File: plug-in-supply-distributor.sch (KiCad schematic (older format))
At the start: 35 parts, among them J1 Conn_02x18_Odd_Even, J2 Conn_02x04_Odd_Even, J3 PV-3, J4 PV-3, J5 PV-3, Q1 2N7002K, Q2 SUD50P04-08, Q3 2N7002K, Q4 SUD50P04-08, U1 74LS27, U2 BD450M5FP

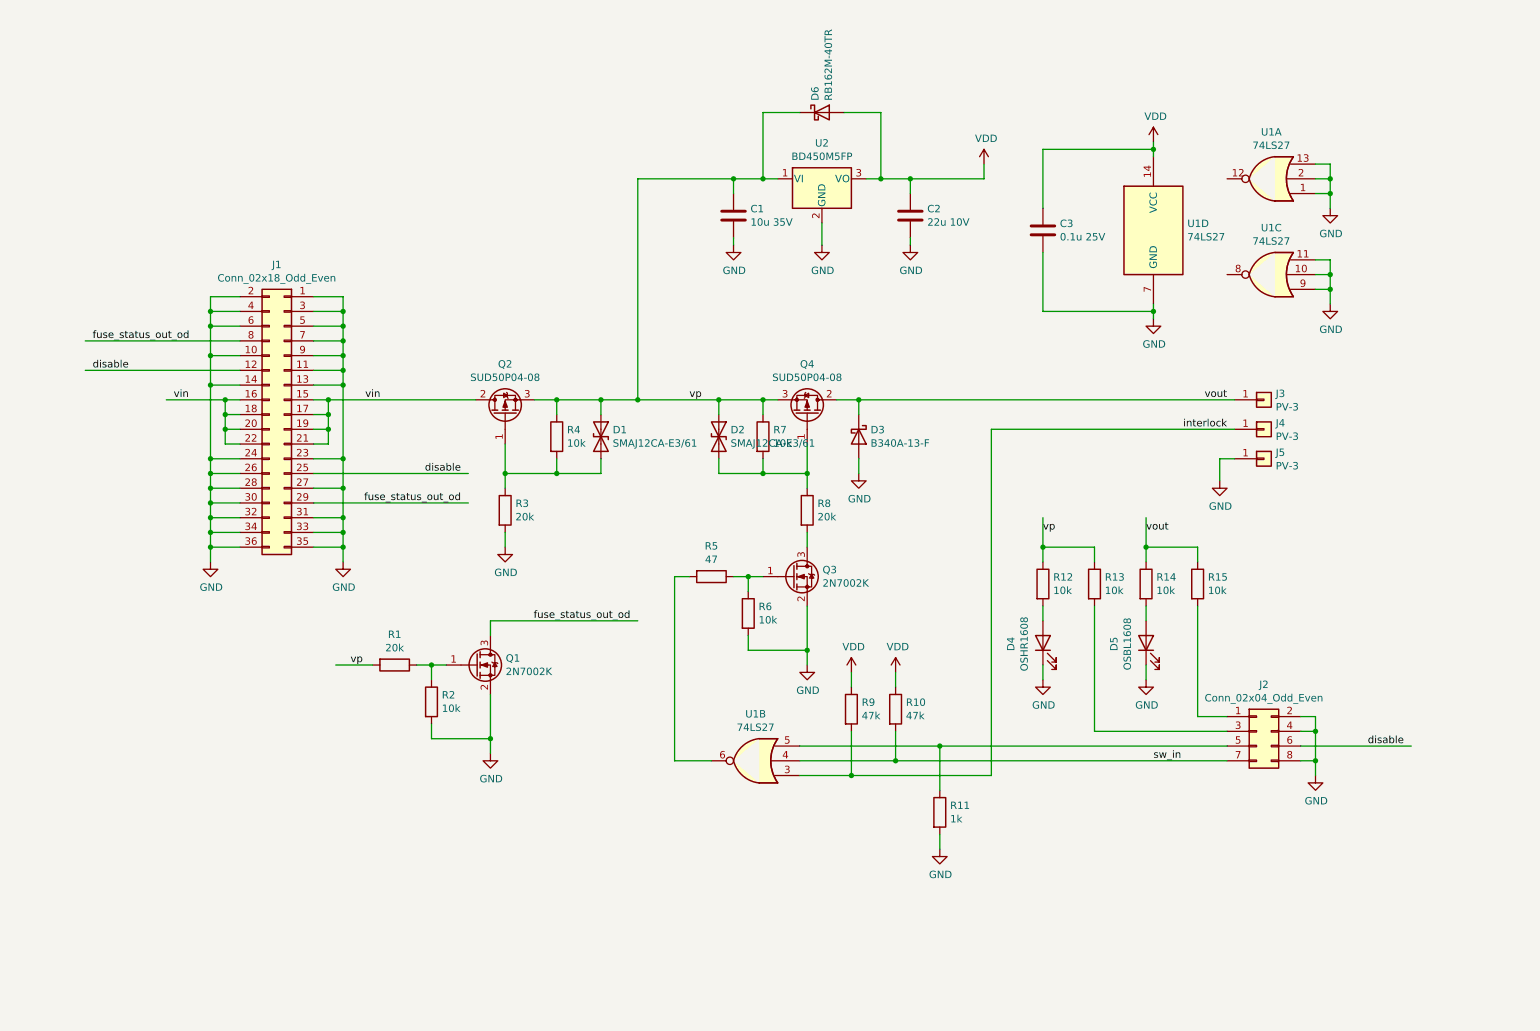
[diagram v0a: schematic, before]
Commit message: Update kicad files
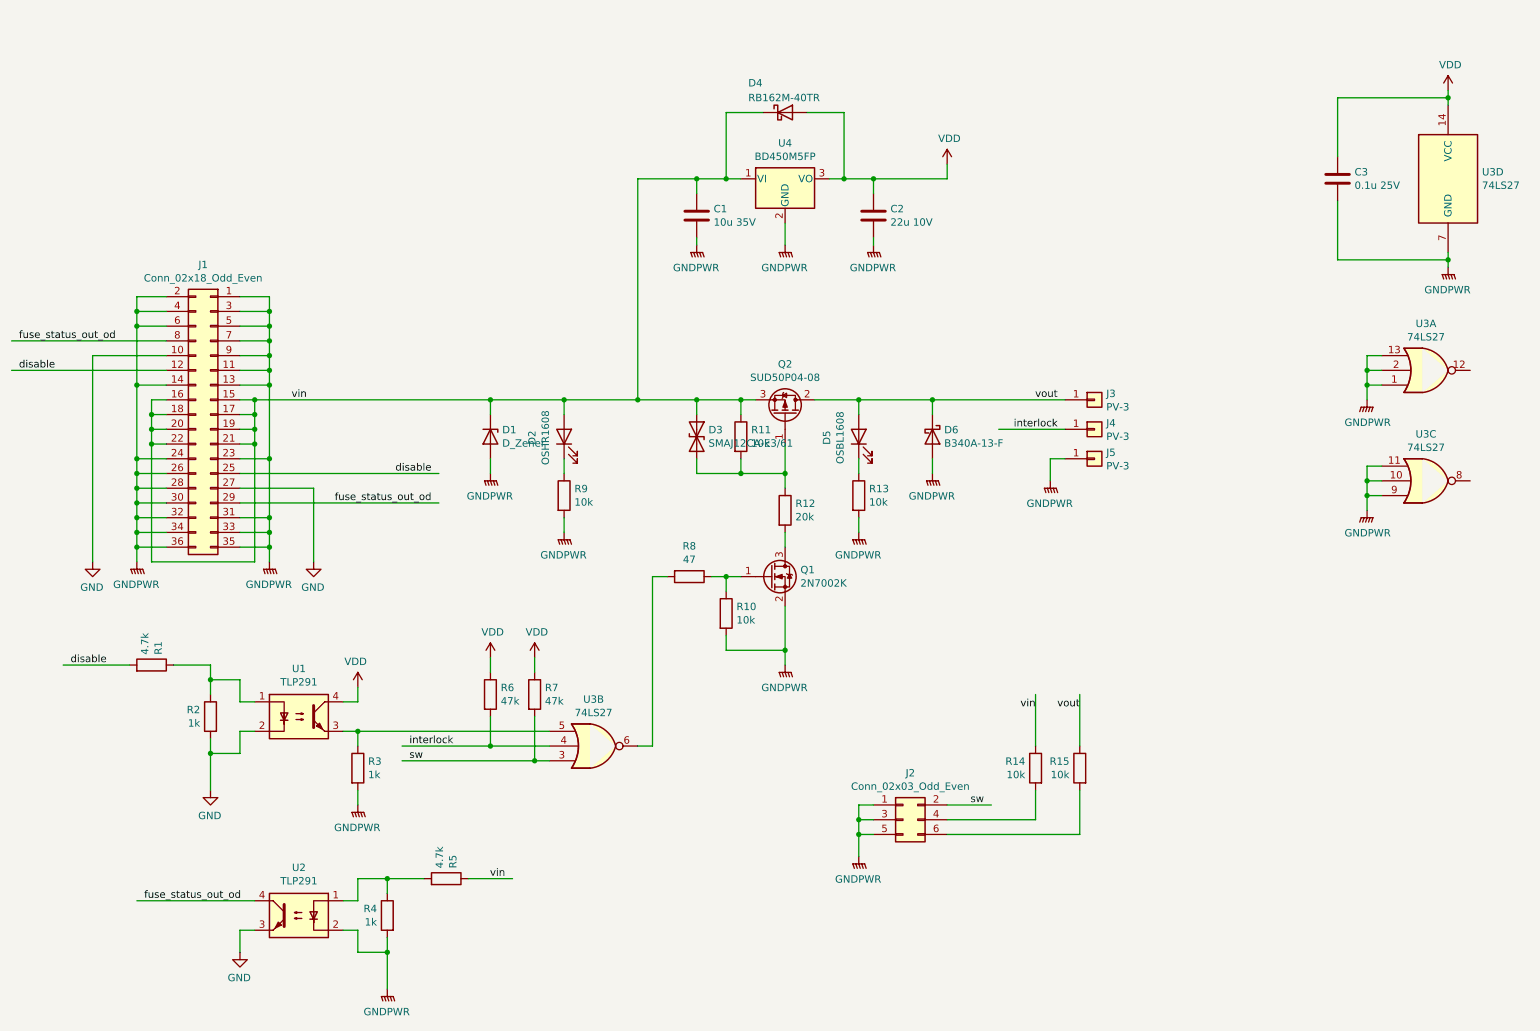
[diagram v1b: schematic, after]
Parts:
- removed D1: SMAJ12CA-E3/61, Diode_SMD:D_SMA, symbol Device:D_TVS
- removed J2: Conn_02x04_Odd_Even, Connector_PinHeader_2.54mm:PinHeader_2x04_P2.54mm_Horizontal, symbol Connector_Generic:Conn_02x04_Odd_Even
- removed Q1: 2N7002K, Package_TO_SOT_SMD:SOT-23, symbol Transistor_FET:2N7002K
- removed Q2: SUD50P04-08, Package_TO_SOT_SMD:TO-252-2, symbol Transistor_FET:SUD50P04-08
- removed R3: 20k, Resistor_SMD:R_0603_1608Metric_Pad1.05x0.95mm_HandSolder, symbol Device:R
- added D1: D_Zener, Diode_SMD:D_SMC, symbol Device:D_Zener
- added J2: Conn_02x03_Odd_Even, Connector_PinHeader_2.54mm:PinHeader_2x03_P2.54mm_Horizontal, symbol Connector_Generic:Conn_02x03_Odd_Even
- added R5: 4.7k, Resistor_SMD:R_0603_1608Metric_Pad1.05x0.95mm_HandSolder, symbol Device:R
- added U1, U2: TLP291, Package_SO:SOIC-4_4.55x2.6mm_P1.27mm, symbol Isolator:TLP291
- R1: value 20k -> 4.7k
- R2, R4: value 10k -> 1k
- renumbered D4 to D2, D2 to D3, D6 to D4, D3 to D6, Q3 to Q1, Q4 to Q2, R6 to R10, R7 to R11, R8 to R12, R14 to R13, R13 to R14, R11 to R3, R10 to R6, R9 to R7, R5 to R8, R12 to R9, U1 to U3, U2 to U4
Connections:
- net labels added: GNDPWR, sw
- net labels removed: sw_in, vp
- wire segments 192 -> 200
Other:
- moved on the sheet: C1, C2, C3, D2, D3, D4, D5, D6, J1, J3, J4, J5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
